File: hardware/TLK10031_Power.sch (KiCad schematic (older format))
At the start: 45 parts, among them U1201 TLK10031

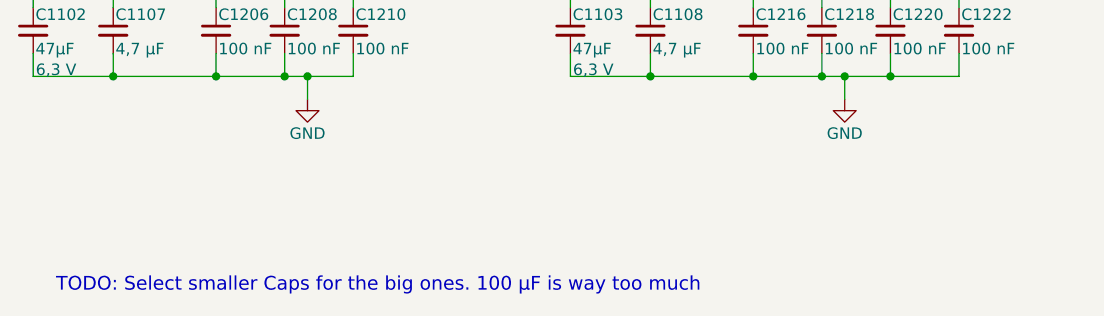
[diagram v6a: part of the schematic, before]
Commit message: Xaui lanes
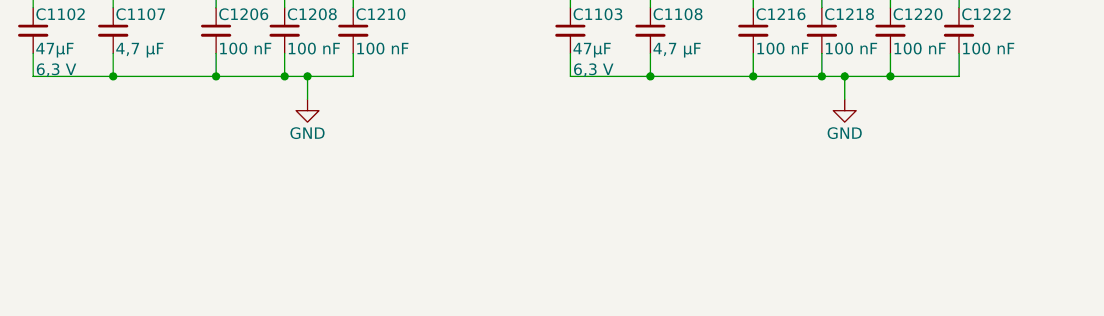
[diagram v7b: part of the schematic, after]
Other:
- note removed: "TODO: Select smaller Caps for the big ones. 100 µF is way too much"
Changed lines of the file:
@@
 Text Notes 7750 6100 0    60   ~ 0
 Layout Note: Place 100 nF Capacitors as close as possible to the Pads
-Text Notes 1050 6950 0    60   ~ 0
-TODO: Select smaller Caps for the big ones. 100 µF is way too much
 Wire Wire Line
 	6450 4150 6750 4150

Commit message: WIP: routing the HF Part of the Camera Connector. I have to move the clock away from the left border.
TODO: Fix DDR3 RAM.
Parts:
- added PO1101, PO1102, PO1103, PO1104, PO1105, PO1106: POWER_OUTPUT, footprints:EMPTY, symbol fixme:POWER_OUTPUT
- R1201, R1202, R1203, R1204, R1205, R1206: footprint Resistors_SMD:R_0603 -> Resistor_SMD:R_0603_1608Metric
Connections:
- wire segments 261 -> 267
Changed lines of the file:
@@
 F 0 "R1201" H 2180 3970 50  0000 L CNN
 F 1 "0" H 2180 3910 50  0000 L CNN
-F 2 "Resistors_SMD:R_0603" H 2150 3950 50  0001 C CNN
+F 2 "Resistor_SMD:R_0603_1608Metric" H 2150 3950 50  0001 C CNN
 F 3 "" H 2150 3950 50  0001 C CNN
 F 4 "1" H 2150 3950 60  0001 C CNN "Populated"
@@
 F 0 "R1202" H 2180 5420 50  0000 L CNN
 F 1 "0" H 2180 5360 50  0000 L CNN
-F 2 "Resistors_SMD:R_0603" H 2150 5400 50  0001 C CNN
+F 2 "Resistor_SMD:R_0603_1608Metric" H 2150 5400 50  0001 C CNN
 F 3 "" H 2150 5400 50  0001 C CNN
 F 4 "1" H 2150 5400 60  0001 C CNN "Populated"
@@
 F 0 "R1204" H 5380 3970 50  0000 L CNN
 F 1 "0" H 5380 3910 50  0000 L CNN
-F 2 "Resistors_SMD:R_0603" H 5350 3950 50  0001 C CNN
+F 2 "Resistor_SMD:R_0603_1608Metric" H 5350 3950 50  0001 C CNN
 F 3 "" H 5350 3950 50  0001 C CNN
 F 4 "1" H 5350 3950 60  0001 C CNN "Populated"
@@
 F 0 "R1206" H 8630 3970 50  0000 L CNN
 F 1 "0" H 8630 3910 50  0000 L CNN
-F 2 "Resistors_SMD:R_0603" H 8600 3950 50  0001 C CNN
+F 2 "Resistor_SMD:R_0603_1608Metric" H 8600 3950 50  0001 C CNN
 F 3 "" H 8600 3950 50  0001 C CNN
 F 4 "1" H 8600 3950 60  0001 C CNN "Populated"
@@
 F 0 "R1203" H 4530 5420 50  0000 L CNN
 F 1 "0" H 4530 5360 50  0000 L CNN
-F 2 "Resistors_SMD:R_0603" H 4500 5400 50  0001 C CNN
+F 2 "Resistor_SMD:R_0603_1608Metric" H 4500 5400 50  0001 C CNN
 F 3 "" H 4500 5400 50  0001 C CNN
 F 4 "1" H 4500 5400 60  0001 C CNN "Populated"
@@
 F 0 "R1205" H 6480 5420 50  0000 L CNN
 F 1 "0" H 6480 5360 50  0000 L CNN
-F 2 "Resistors_SMD:R_0603" H 6450 5400 50  0001 C CNN
+F 2 "Resistor_SMD:R_0603_1608Metric" H 6450 5400 50  0001 C CNN
 F 3 "" H 6450 5400 50  0001 C CNN
 F 4 "1" H 6450 5400 60  0001 C CNN "Populated"
@@
 	4500 4150 4950 4150
 Wire Wire Line
-	4950 4150 5250 4150
+	4950 4150 5150 4150
 Wire Wire Line
 	5250 4150 5350 4150
@@
 	1300 5600 1750 5600
 Wire Wire Line
-	1750 5600 2050 5600
+	1750 5600 1950 5600
 Wire Wire Line
 	2050 5600 2150 5600
@@
 	2050 4150 2150 4150
 Wire Wire Line
-	2350 4150 2650 4150
+	2350 4150 2450 4150
 Wire Wire Line
 	2650 4150 2950 4150
@@
 	7750 4150 8200 4150
 Wire Wire Line
-	8200 4150 8500 4150
+	8200 4150 8400 4150
 Wire Wire Line
 	8500 4150 8600 4150
@@
 	3650 5600 4100 5600
 Wire Wire Line
-	4100 5600 4400 5600
+	4100 5600 4300 5600
 Wire Wire Line
 	4400 5600 4500 5600
@@
 	3650 6000 4100 6000
 Wire Wire Line
-	6200 5600 6450 5600
+	6200 5600 6350 5600
 Wire Wire Line
 	6650 5600 6950 5600
@@
 	1    0    0    -1
 $EndComp
+$Comp
+L fixme:POWER_OUTPUT PO1102
+U 1 1 5BECD986
+P 2450 4050
+F 0 "PO1102" H 2450 4050 50  0001 C CNN
+F 1 "POWER_OUTPUT" H 2450 4200 50  0001 C CNN
+F 2 "footprints:EMPTY" H 2450 4050 50  0001 C CNN
+F 3 "" H 2450 4050 50  0001 C CNN
+	1    2450 4050
+	1    0    0    -1
+$EndComp
+Connection ~ 2450 4150
+Wire Wire Line
+	2450 4150 2650 4150
+$Comp
+L fixme:POWER_OUTPUT PO1101
+U 1 1 5BECDB2F
+P 1950 5500
+F 0 "PO1101" H 1950 5500 50  0001 C CNN
+F 1 "POWER_OUTPUT" H 1950 5650 50  0001 C CNN
+F 2 "footprints:EMPTY" H 1950 5500 50  0001 C CNN
+F 3 "" H 1950 5500 50  0001 C CNN
+	1    1950 5500
+	1    0    0    -1
+$EndComp
+Connection ~ 1950 5600
+Wire Wire Line
+	1950 5600 2050 5600
+$Comp
+L fixme:POWER_OUTPUT PO1103
+U 1 1 5BECDCA4
+P 4300 5500
+F 0 "PO1103" H 4300 5500 50  0001 C CNN
+F 1 "POWER_OUTPUT" H 4300 5650 50  0001 C CNN
+F 2 "footprints:EMPTY" H 4300 5500 50  0001 C CNN
+F 3 "" H 4300 5500 50  0001 C CNN
+	1    4300 5500
+	1    0    0    -1
+$EndComp
+Connection ~ 4300 5600
+Wire Wire Line
+	4300 5600 4400 5600
+$Comp
+L fixme:POWER_OUTPUT PO1104
+U 1 1 5BECDEFA
+P 5150 4050
+F 0 "PO1104" H 5150 4050 50  0001 C CNN
+F 1 "POWER_OUTPUT" H 5150 4200 50  0001 C CNN
+F 2 "footprints:EMPTY" H 5150 4050 50  0001 C CNN
+F 3 "" H 5150 4050 50  0001 C CNN
+	1    5150 4050
+	1    0    0    -1
+$EndComp
+Connection ~ 5150 4150
+Wire Wire Line
+	5150 4150 5250 4150
+$Comp
+L fixme:POWER_OUTPUT PO1105
+U 1 1 5BECE1AA
+P 6350 5500
+F 0 "PO1105" H 6350 5500 50  0001 C CNN
+F 1 "POWER_OUTPUT" H 6350 5650 50  0001 C CNN
+F 2 "footprints:EMPTY" H 6350 5500 50  0001 C CNN
+F 3 "" H 6350 5500 50  0001 C CNN
+	1    6350 5500
+	1    0    0    -1
+$EndComp
+Connection ~ 6350 5600
+Wire Wire Line
+	6350 5600 6450 5600
+$Comp
+L fixme:POWER_OUTPUT PO1106
+U 1 1 5BECE4B4
+P 8400 4050
+F 0 "PO1106" H 8400 4050 50  0001 C CNN
+F 1 "POWER_OUTPUT" H 8400 4200 50  0001 C CNN
+F 2 "footprints:EMPTY" H 8400 4050 50  0001 C CNN
+F 3 "" H 8400 4050 50  0001 C CNN
+	1    8400 4050
+	1    0    0    -1
+$EndComp
+Connection ~ 8400 4150
+Wire Wire Line
+	8400 4150 8500 4150
 $EndSCHEMATC
